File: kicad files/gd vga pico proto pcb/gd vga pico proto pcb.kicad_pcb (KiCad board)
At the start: 2 copper layers, 66 x 66 mm, 62 parts, among them J1 RGB Bin, J2 CLKS, J3 SWD, J4 L77HDE15SD1CH4F, J5 VID_TXRX, J6 WIN, J7 5V, J8 USB_B_Micro, SW1 2040 RESET, U1 RP2040, U2 74HCT245, U3 74LVC2G04, U4 74LVC2G04, U5 MIC5504-3.3YM5, U6 74LVC2G04-DNP, Y1 ECS-120-18-33-JEM-TR

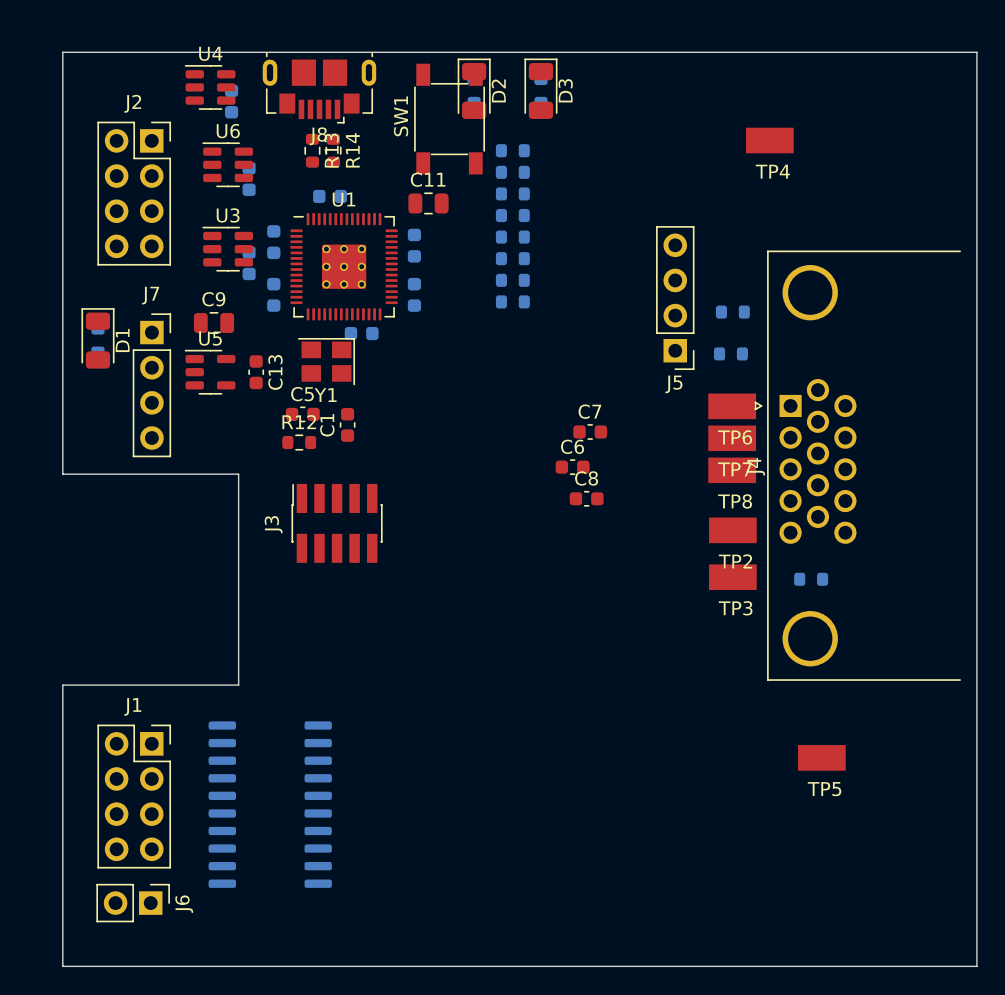
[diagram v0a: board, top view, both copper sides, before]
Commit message: rev1 finish from stream, need final review
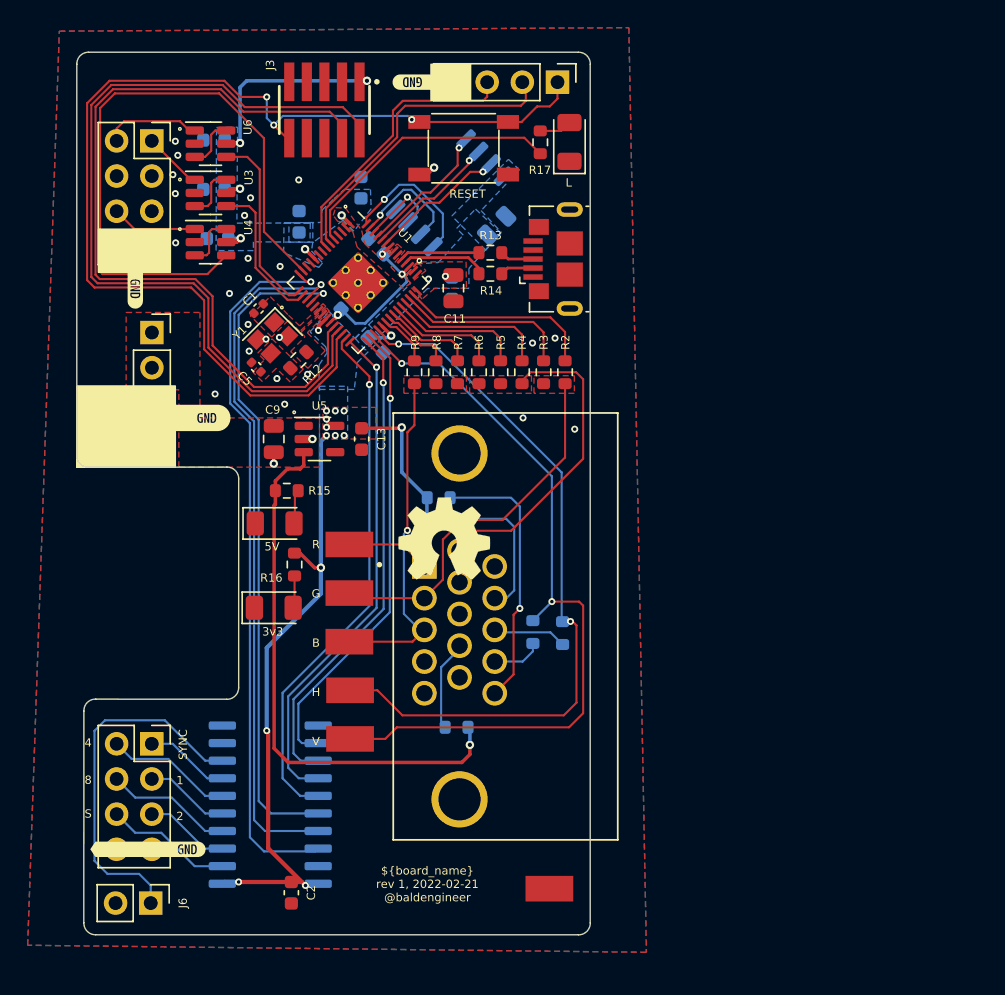
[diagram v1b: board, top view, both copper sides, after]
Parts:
- removed C15: 1u, Capacitor_SMD:C_0603_1608Metric
- removed C7: 100n, Capacitor_SMD:C_0603_1608Metric
- added C18: 100n, Capacitor_SMD:C_0805_2012Metric, B.Cu at (105.0, 55.7)
- added REF**: OSHW-Symbol_6.7x6mm_SilkScreen, Symbol:OSHW-Symbol_6.7x6mm_SilkScreen, F.Cu at (101.2, 78.3)
- added REF**: OSHW-Symbol_6.7x6mm_SilkScreen, Symbol:OSHW-Symbol_6.7x6mm_SilkScreen, B.Cu at (107.9, 95.6)
- added U7: W25Q128JVS, Package_SO:SOIC-8_5.23x5.23mm_P1.27mm, B.Cu at (101.6, 53.3)
- added kibuzzard-62146889: G***, kibuzzard-62146889, F.Cu at (79.8, 100.8)
- added kibuzzard-62146889: G***, kibuzzard-62146889, B.Cu at (79.8, 100.8)
- added kibuzzard-621468FD: G***, kibuzzard-621468FD, F.Cu at (81.3, 69.6)
- added kibuzzard-621468FD: G***, kibuzzard-621468FD, B.Cu at (81.3, 69.6)
- added kibuzzard-621469E6: G***, kibuzzard-621469E6, F.Cu at (78.9, 59.5)
- added kibuzzard-621469E6: G***, kibuzzard-621469E6, F.Cu at (99.7, 45.3)
- added kibuzzard-621469E6: G***, kibuzzard-621469E6, B.Cu at (99.7, 45.4)
- added kibuzzard-621469E6: G***, kibuzzard-621469E6, B.Cu at (78.8, 59.4)
- C1, C5: value 27p -> 6p; footprint Capacitor_SMD:C_0603_1608Metric -> Capacitor_SMD:C_0402_1005Metric
- C2, R15, R16, R17, R2, R3, R4, R5, R6, R7, R8, R9: moved to F.Cu
- C6: value 100n -> 1u; moved to B.Cu
- C8: moved to B.Cu
- J3: footprint Connector_PinSocket_1.27mm:PinSocket_2x05_P1.27mm_Vertical_SMD -> FTSH-105-01-L-DV-K:SAMTEC_FTSH-105-XX-X-DV
- J4: footprint Connector_Dsub:DSUB-15-HD_Female_Horizontal_P2.29x1.98mm_EdgePinOffset8.35mm_Housed_MountingHolesOffset10.89mm -> L77HDE15SD1CH4F:AMPHENOL_L77HDE15SD1CH4F
- Y1: value ECS-120-18-33-JEM-TR -> ABM10AIG-12.000MHZ-7-D2Z-T; footprint Crystal:Crystal_SMD_3225-4Pin_3.2x2.5mm -> Crystal:Crystal_SMD_2520-4Pin_2.5x2.0mm
- moved TP4 52.5 mm to (76.7, 70.7), turned to 90 degrees
- moved C2 43.2 mm to (90.2, 103.9)
- moved D2 40.0 mm to (88.9, 83.3), turned to 0 degrees
- moved R16 36.6 mm to (90.4, 80.2)
- moved TP8 30.3 mm to (94.4, 85.8)
- moved TP3 30.0 mm to (94.4, 92.8)
- moved TP2 30.0 mm to (94.4, 89.3)
- moved J3 29.9 mm to (92.6, 47.3), turned to 180 degrees
- moved TP7 29.8 mm to (94.4, 82.3)
- moved TP6 29.4 mm to (94.4, 78.7)
- moved J4 28.7 mm to (102.3, 84.7)
- moved R1 27.8 mm to (102.1, 91.9)
- moved RNP2 25.1 mm to (100.8, 75.4)
- moved RNP1 24.3 mm to (100.8, 76.9)
- moved C8 22.3 mm to (94.3, 61.2), turned to 45 degrees
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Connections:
- J5 pad 1: /VIN_EN -> /VID_EN
- U1 pad 11: /HSYNC -> unconnected-(U1-Pad11)
- U1 pad 12: /VSYNC -> unconnected-(U1-Pad12)
- U1 pad 13: /LED_L -> /~{RESET_RP}
- U1 pad 14: unconnected-(U1-Pad14) -> /SERVID_RP
- U1 pad 15: unconnected-(U1-Pad15) -> /7M_RP
- U1 pad 16: unconnected-(U1-Pad16) -> /14M_RP
- U1 pad 17: /VGA_SDA -> /RGB2_RP
- U1 pad 18: /VGA_SCL -> /RGB1_RP
- U1 pad 2: /RED0 -> unconnected-(U1-Pad2)
- U1 pad 27: /VID_TX -> /RGB8_RP
- U1 pad 28: /VID_RX -> /RGB4_RP
- U1 pad 29: /~{WINDOW_RP} -> /~{SYNC_RP}
- U1 pad 3: /RED1 -> unconnected-(U1-Pad3)
- U1 pad 30: /~{SYNC_RP} -> /~{WINDOW_RP}
- U1 pad 31: /7M_RP -> /VSYNC
- U1 pad 32: /14M_RP -> /HSYNC
- U1 pad 34: /RGB1_RP -> /BLU2
- U1 pad 35: /RGB2_RP -> /BLU1
- U1 pad 36: /RGB4_RP -> /BLU0
- U1 pad 37: /RGB8_RP -> /GRN2
- U1 pad 38: /SERVID_RP -> /GRN1
- U1 pad 39: unconnected-(U1-Pad39) -> /GRN0
- U1 pad 4: /GRN0 -> unconnected-(U1-Pad4)
- U1 pad 40: unconnected-(U1-Pad40) -> /RED1
- U1 pad 41: unconnected-(U1-Pad41) -> /RED0
- U1 pad 5: /GRN1 -> /LED_L
- U1 pad 6: /GRN2 -> /VID_TX
- U1 pad 7: /BLU0 -> /VID_RX
- U1 pad 8: /BLU1 -> unconnected-(U1-Pad8)
- U1 pad 9: /BLU2 -> unconnected-(U1-Pad9)
- U2 pad 1: +5V -> +3V3
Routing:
- net +3V3: track 0.00 -> 81.0 mm, vias 0 -> 23
- net /VID_EN: track 0.00 -> 80.5 mm, vias 0 -> 3
- net /SWDIO: track 0.00 -> 61.0 mm
- net /SWCLK: track 0.00 -> 58.4 mm
- net /VSYNC: track 0.00 -> 55.9 mm, vias 0 -> 2
- net /HSYNC: track 0.00 -> 52.7 mm, vias 0 -> 2
- net /SERVID_RP: track 0.00 -> 51.8 mm, vias 0 -> 1
- net /RGB2_RP: track 0.00 -> 50.7 mm, vias 0 -> 1
- net /RGB1_RP: track 0.00 -> 48.3 mm, vias 0 -> 1
- net /~{RESET_RP}: track 0.00 -> 45.9 mm
- net +5V: track 0.00 -> 39.6 mm, vias 0 -> 1
- net /RGB8_RP: track 0.00 -> 38.5 mm, vias 0 -> 1
- net /RGB4_RP: track 0.00 -> 36.7 mm, vias 0 -> 1
- net /~{SYNC_RP}: track 0.00 -> 35.0 mm, vias 0 -> 1
- net /~{WINDOW_RP}: track 0.00 -> 33.9 mm, vias 0 -> 1
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- added copper zone on B.Cu, net +3V3
- added copper zone on F.Cu, net +3V3
- added copper zone on F.Cu, net +5V
- added copper zone on F.Cu, net /VGA_B
- added copper zone on F.Cu, net /VGA_G
- added copper zone on F.Cu, net /VGA_R
- added copper zone on F.Cu, net /XIN
- added copper zone on F.Cu, net /XOUT
- added copper zone on B.Cu, net GND
- added copper zone on F.Cu, net GND
- added copper zone on F.Cu, net Net-(C5-Pad1)
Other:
- board size 66 x 66 mm -> 37.1 x 63.8 mm
- rule pad_to_mask_clearance: 0 -> 0.0508
- board text added: "${board_name} rev ${REVISION}, ${ISSUE_DATE} @baldengineer"
- board text added: "1"
- board text added: "2"
- board text added: "3v3"
- board text added: "4"
- board text added: "5V"
- board text added: "8"
- board text added: "B"
- board text added: "G"
- board text added: "H"
- board text added: "L"
- board text added: "R"
- board text added: "RESET"
- board text added: "S"
- board text added: "SYNC"
- board text added: "V"
